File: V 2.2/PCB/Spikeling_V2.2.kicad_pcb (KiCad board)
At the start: 2 copper layers, 120 x 80 mm, 51 parts

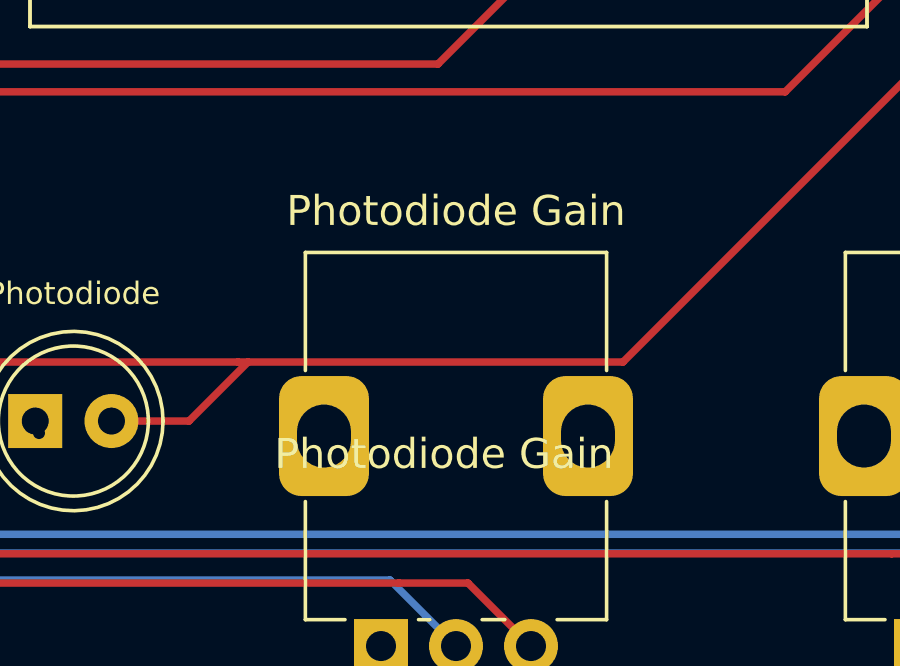
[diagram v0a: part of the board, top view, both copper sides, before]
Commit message: update pcb
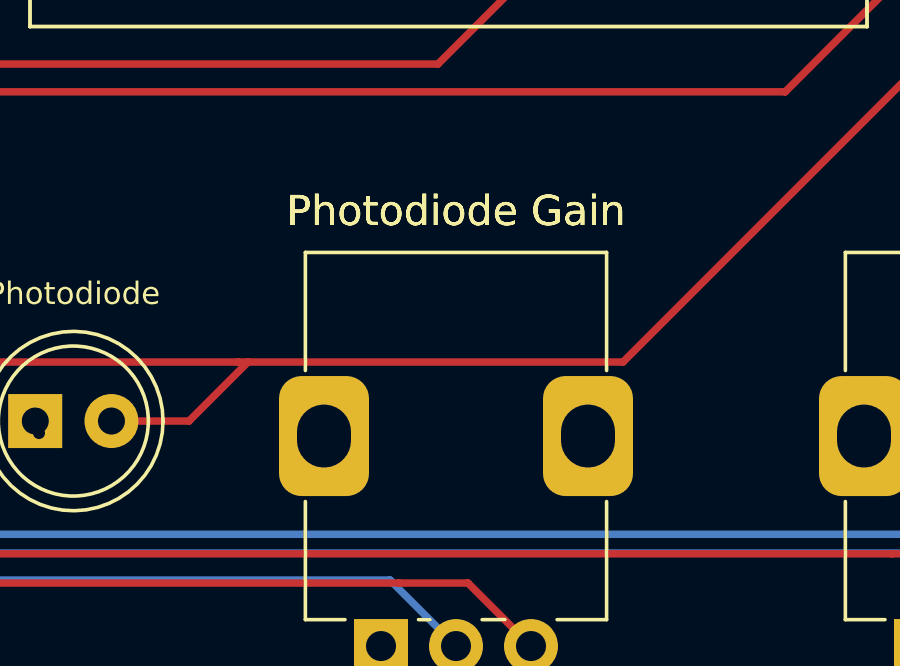
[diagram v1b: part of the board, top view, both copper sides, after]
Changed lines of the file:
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@@
   (footprint "Audio_Module:Spikeling_Photoreceptor" (layer "F.Cu")
     (at 159.6 122.9)
-    (fp_text reference "Photodiode Gain" (at 0 -0.5 unlocked) (layer "F.SilkS")
+    (fp_text reference "Photodiode Gain" (at 0.4 -8.6 unlocked) (layer "F.SilkS")
       (effects (font (size 1 1) (thickness 0.15)))
     )
